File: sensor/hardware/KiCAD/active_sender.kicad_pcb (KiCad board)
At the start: 2 copper layers, 83 x 80 mm, 29 parts, among them J1 220V0, J2 Buzzer, J3 Water Sensor, Q1 AO3400A, SW1 SW_Push, SW2 SW_SPDT, U1 ESP32-C3_SUPERMINI_TH, U2 Ai-Thinker-Ra-02, U3 HLK-PM12

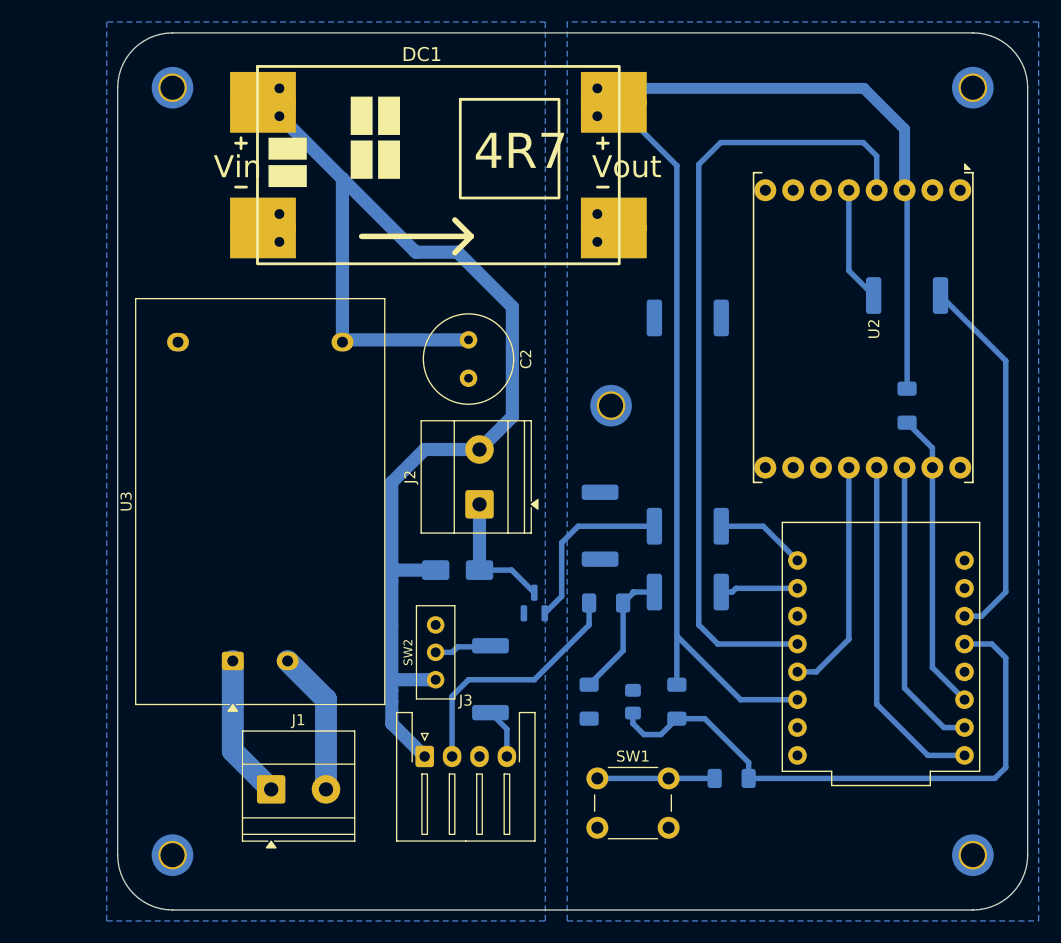
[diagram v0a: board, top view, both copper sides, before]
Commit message: sensor iteration 2
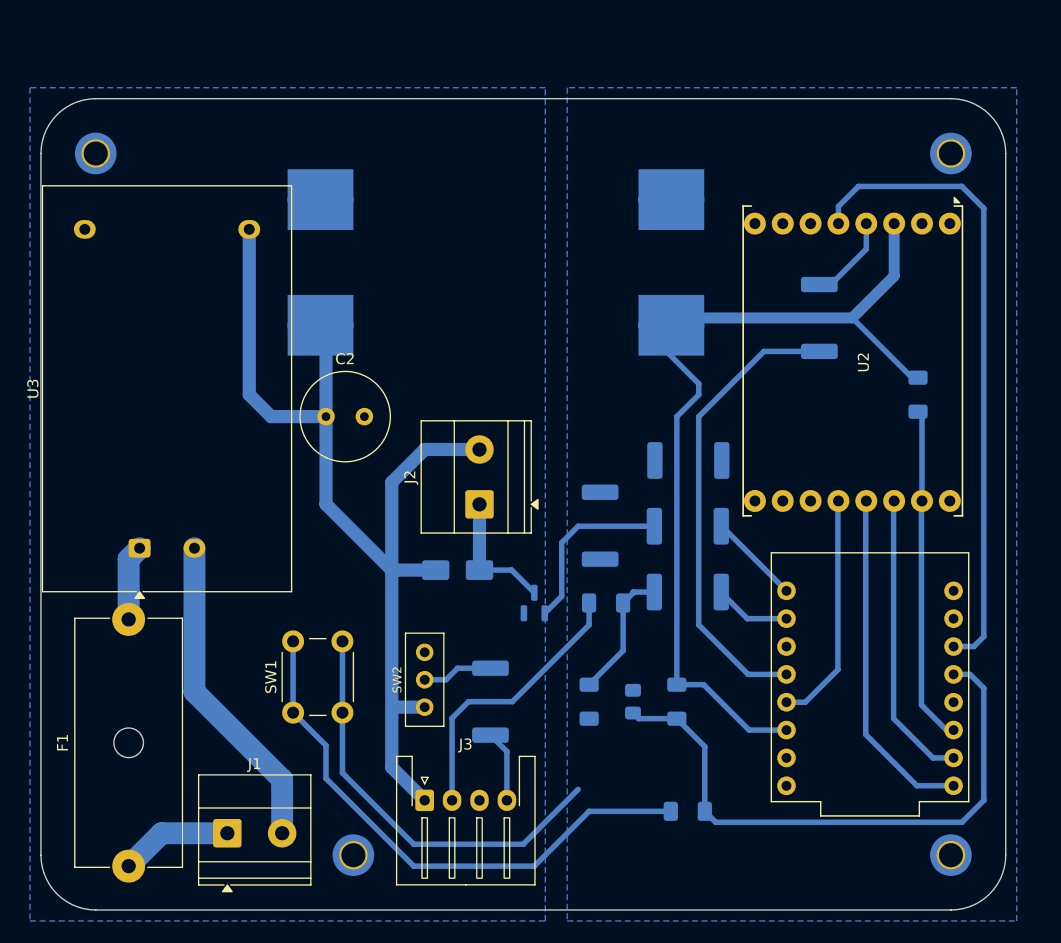
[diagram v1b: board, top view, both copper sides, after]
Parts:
- removed R9: 0R, Resistor_SMD:R_2512_6332Metric_Pad1.40x3.35mm_HandSolder
- removed the REF** at (108.0, 82.0)
- added F1: Fuse, Fuse:Fuseholder_Cylinder-5x20mm_Schurter_0031_8201_Horizontal_Open, F.Cu at (64.0, 124.0)
- added R13: 0R, Resistor_SMD:R_2512_6332Metric_Pad1.40x3.35mm_HandSolder, B.Cu at (127.0, 74.0)
- DC1: moved to B.Cu
- moved SW1 28.4 mm to (79.0, 110.0), turned to 90 degrees
- moved DC1 27.4 mm to (81.0, 77.9)
- moved REF** 16.5 mm to (84.5, 123.0)
- moved C2 14.8 mm to (82.0, 83.0), turned to 0 degrees
- moved U3 13.3 mm to (65.0, 95.0)
- moved R11 13.0 mm to (115.0, 87.0)
- moved REF** 9.22 mm to (61.0, 59.0)
- moved REF** 6.32 mm to (139.0, 59.0)
- moved J1 5.66 mm to (73.0, 121.0)
- moved R4 5.00 mm to (115.0, 119.0)
- moved J3 4.00 mm to (91.0, 118.0)
- moved U2 3.19 mm to (130.1, 78.0)
- moved U1 2.94 mm to (131.6, 106.8)
- moved SW2 2.69 mm to (91.0, 107.0)
- moved R10 2.05 mm to (97.0, 109.0)
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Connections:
- J1 pad 1: /220V0 -> Net-(J1-Pin_1)
- U2 pad 4: /LORA_RESET -> Net-(U2-~{RESET})
- U2 pad 5: Net-(U2-DIO0) -> /LORA_DIO0
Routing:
- net Net-(R4-Pad2): track 11.0 -> 50.6 mm
- net +3.3V: track 123.2 -> 84.1 mm
- net GNDD: track 0.00 -> 38.3 mm
- net /LORA_RESET: track 72.4 -> 42.3 mm
- net /LORA_DIO0: track 34.2 -> 58.6 mm
- net /12V0: track 114.8 -> 92.9 mm
- net /N 220V0: track 13.2 -> 29.3 mm
- net Net-(U2-DIO0): track 10.5 -> 0.00 mm
- net Net-(J1-Pin_1): track 0.00 -> 10.2 mm
- net Net-(U2-~{RESET}): track 0.00 -> 6.89 mm
- net /220V0: track 13.2 -> 6.91 mm
- net /LORA_NSS: track 27.4 -> 30.8 mm
- net Net-(J3-Pin_2): track 22.7 -> 25.5 mm
- net /MODE: track 4.62 -> 6.57 mm
- net Net-(SW2-B): track 5.25 -> 6.43 mm
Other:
- board size 83 x 80 mm -> 88 x 74 mm
